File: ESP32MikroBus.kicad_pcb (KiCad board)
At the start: 4 copper layers, 30.2 x 44.5 mm, 27 parts, among them IC1 ESP32-C6-WROOM-1-N4, IC2 AP7361C-33ER-13, J1 USB4105GFA120, J2 CON_HDR_MIKROBUS_SOCKET_TH, J3 Qwiic, U1 USBLC6-2P6

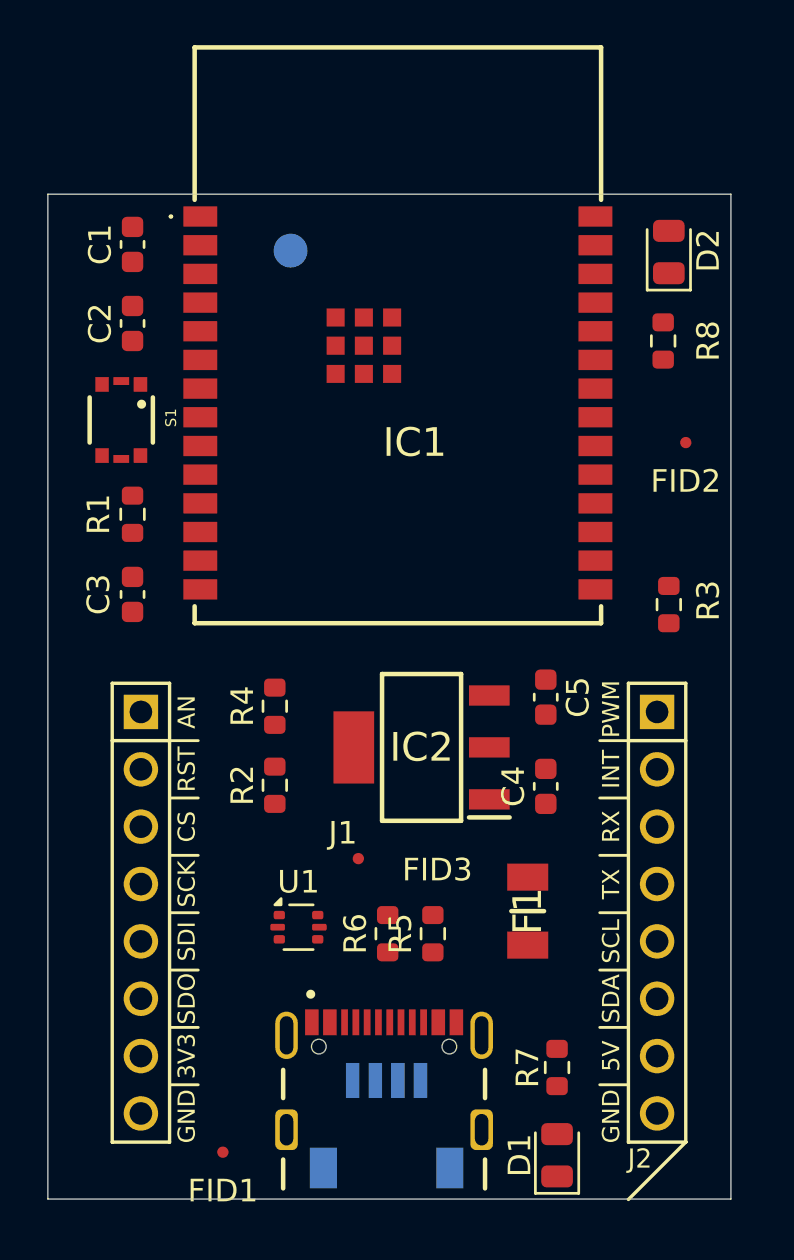
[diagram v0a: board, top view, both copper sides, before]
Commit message: PCB Layout v1.0 ready for verification by PCBWay
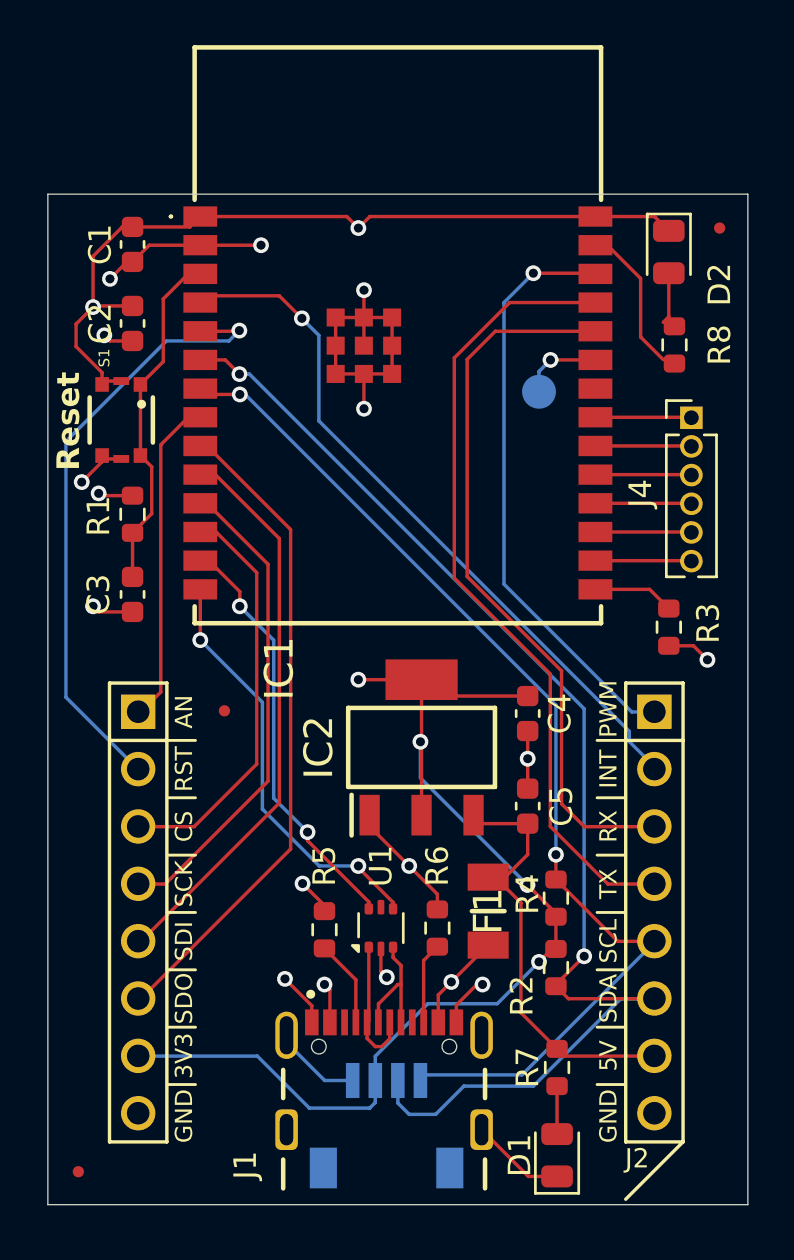
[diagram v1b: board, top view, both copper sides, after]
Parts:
- added G***: OpenSourceHardware_Logo, tecnova:OpenSourceHardware_Logo, B.Cu at (35.8, 43.3)
- added G***: LOGO, tecnova:Tecnova_logo, B.Cu at (54.7, 42.8)
- added G***: MikroBus_Logo, tecnova:MikroBus_Logo, B.Cu at (43.8, 63.2)
- added J4: Conn_01x06, Connector_PinHeader_1.27mm:PinHeader_1x06_P1.27mm_Vertical, F.Cu at (57.2, 47.4)
- moved R4 15.1 mm to (51.2, 68.7)
- moved R2 14.8 mm to (51.2, 71.8), turned to -90 degrees
- moved TP1 12.7 mm to (50.5, 46.2)
- moved FID2 9.62 mm to (58.5, 39.0)
- moved FID3 8.83 mm to (36.6, 60.4)
- moved FID1 6.46 mm to (30.1, 80.8)
- moved C5 4.89 mm to (50.0, 64.6), turned to 90 degrees
- moved R5 4.80 mm to (41.0, 70.1)
- moved U1 3.65 mm to (43.5, 70.0), turned to 90 degrees
- moved C4 3.32 mm to (50.0, 60.5), turned to -90 degrees
- moved R6 2.21 mm to (46.0, 70.0)
- moved F1 1.75 mm to (48.2, 69.2), turned to -90 degrees
- moved R3 1.00 mm to (56.2, 56.7)
- moved R8 0.53 mm to (56.5, 44.2)
- moved J2 0.12 mm to (44.2, 69.3)
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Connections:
- C5 pad 1: Net-(IC2-IN) -> +5V
- F1 pad 1: +VBUS -> +5V
- F1 pad 2: +5V -> +VBUS
- IC1 pad 10: unconnected-(IC1-IO8-Pad10) -> /MB_MISO
- IC1 pad 11: unconnected-(IC1-IO10-Pad11) -> /MB_SCK
- IC1 pad 12: unconnected-(IC1-IO11-Pad12) -> /MB_CS
- IC1 pad 16: unconnected-(IC1-IO18-Pad16) -> /SPARE6
- IC1 pad 17: unconnected-(IC1-IO19-Pad17) -> /SPARE5
- IC1 pad 18: unconnected-(IC1-IO20-Pad18) -> /SPARE4
- IC1 pad 19: unconnected-(IC1-IO21-Pad19) -> /SPARE3
- IC1 pad 20: unconnected-(IC1-IO22-Pad20) -> /SPARE2
- IC1 pad 21: unconnected-(IC1-IO23-Pad21) -> /SPARE1
- IC1 pad 26: unconnected-(IC1-IO3-Pad26) -> /MB_PWM
- IC1 pad 27: unconnected-(IC1-IO2-Pad27) -> /USR_LED
- IC1 pad 4: unconnected-(IC1-IO4-Pad4) -> /MB_INT
- IC1 pad 5: unconnected-(IC1-IO5-Pad5) -> /MB_RST
- IC1 pad 9: unconnected-(IC1-IO1-Pad9) -> /MB_MOSI
- IC2 pad 3: Net-(IC2-IN) -> +5V
- J2 pad 15: Net-(J2-+5V) -> +5V
- R3 pad 1: +3V3 -> +3.3V
- R7 pad 1: Net-(R7-Pad1) -> +5V
- S1 pad 4: Net-(S1-Pad4) -> GND
- S1 pad 6: Net-(S1-Pad4) -> GND
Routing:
- net GND: track 0.00 -> 78.3 mm, vias 0 -> 12
- net +3.3V: track 0.00 -> 61.1 mm, vias 0 -> 9
- net /I2C_SDA: track 0.00 -> 55.7 mm, vias 0 -> 2
- net /I2C_SCL: track 0.00 -> 47.9 mm, vias 0 -> 2
- net /TXD: track 0.00 -> 35.6 mm
- net /RXD: track 0.00 -> 32.3 mm
- net /MB_INT: track 0.00 -> 31.5 mm, vias 0 -> 1
- net /MB_MOSI: track 0.00 -> 29.1 mm
- net /MB_RST: track 0.00 -> 27.4 mm, vias 0 -> 1
- net /MB_PWM: track 0.00 -> 26.2 mm, vias 0 -> 1
- net /MB_MISO: track 0.00 -> 25.1 mm
- net /MB_SCK: track 0.00 -> 21.2 mm
- net +5V: track 0.00 -> 19.4 mm
- net /USB_D_MIN: track 0.00 -> 18.7 mm, vias 0 -> 2
- net /USB_D_PLUS: track 0.00 -> 18.7 mm, vias 0 -> 2
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- added copper zone on In2.Cu, net +3.3V
- added copper zone on In2.Cu, net +VBUS
- added copper zone on In1.Cu, net GND
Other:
- board size 30.2 x 44.5 mm -> 31 x 44.8 mm
- board text added: "ESP32C6 + mikroBUS v1.0"
- board text added: "Reset"
